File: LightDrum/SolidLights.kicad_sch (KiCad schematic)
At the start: 11 parts, among them U12 NCR420PAS, U13 NCR420PAS, U14 NCR420PAS, U15 INA180A2

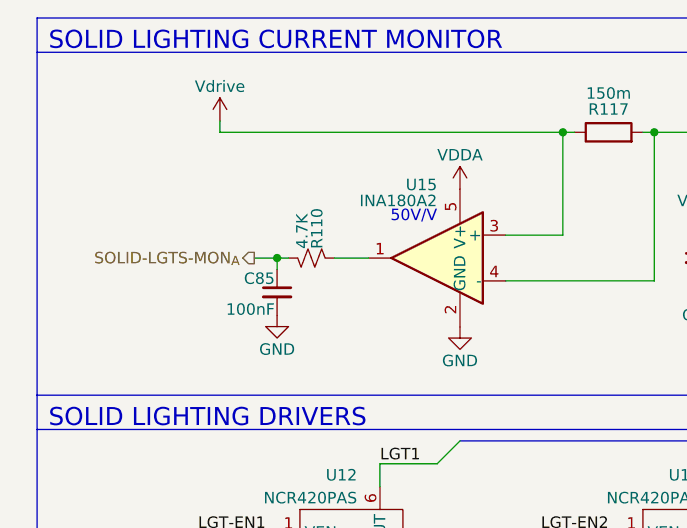
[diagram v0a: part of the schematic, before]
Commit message: REV13 - Update to KiCAD 8
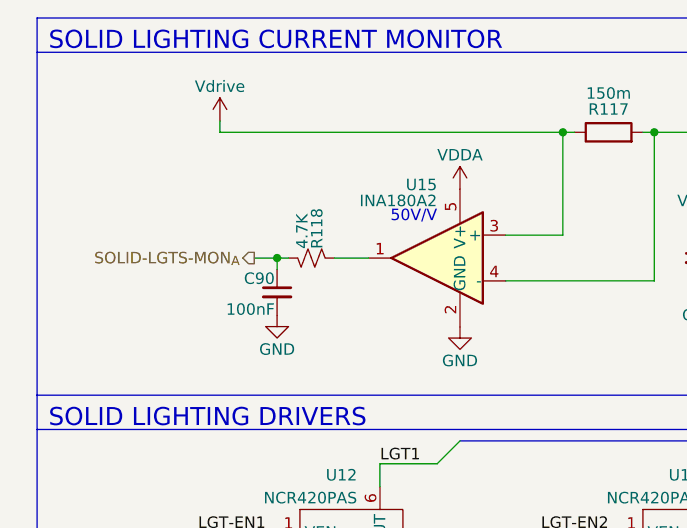
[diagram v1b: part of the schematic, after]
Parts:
- renumbered C85 to C90, R110 to R118

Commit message: REV13 - Revert to KiCAD 7
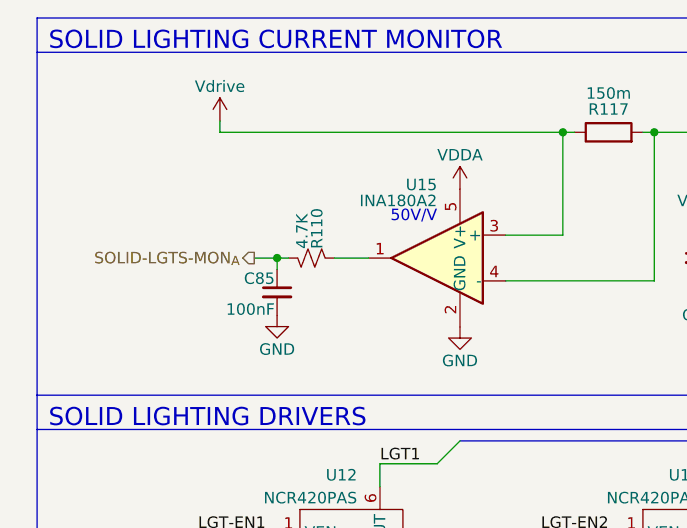
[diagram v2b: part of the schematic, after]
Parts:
- renumbered C90 to C85, R118 to R110
